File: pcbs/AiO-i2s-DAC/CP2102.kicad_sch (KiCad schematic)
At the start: 12 parts, among them U3 CP2102-GM

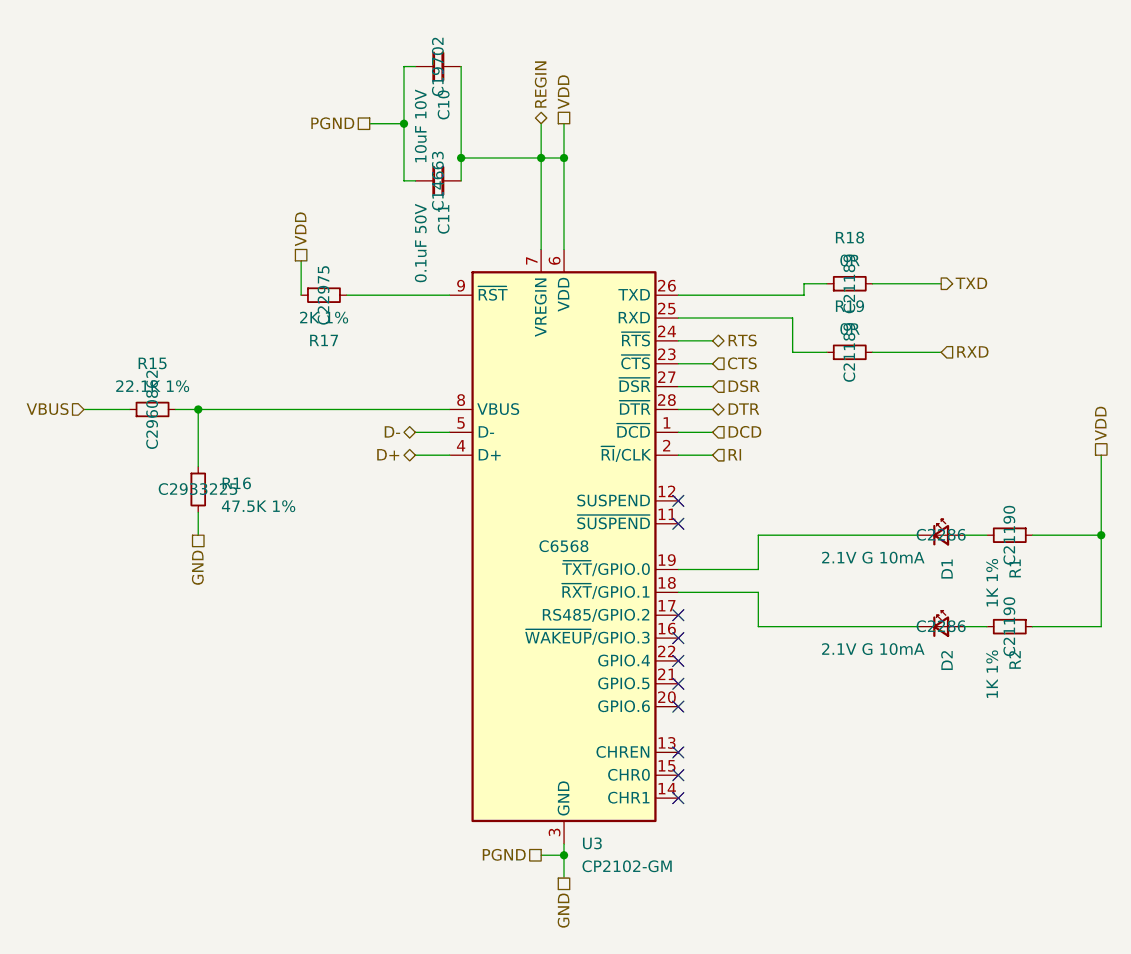
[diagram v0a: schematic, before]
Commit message: LCSC BOM Preparation
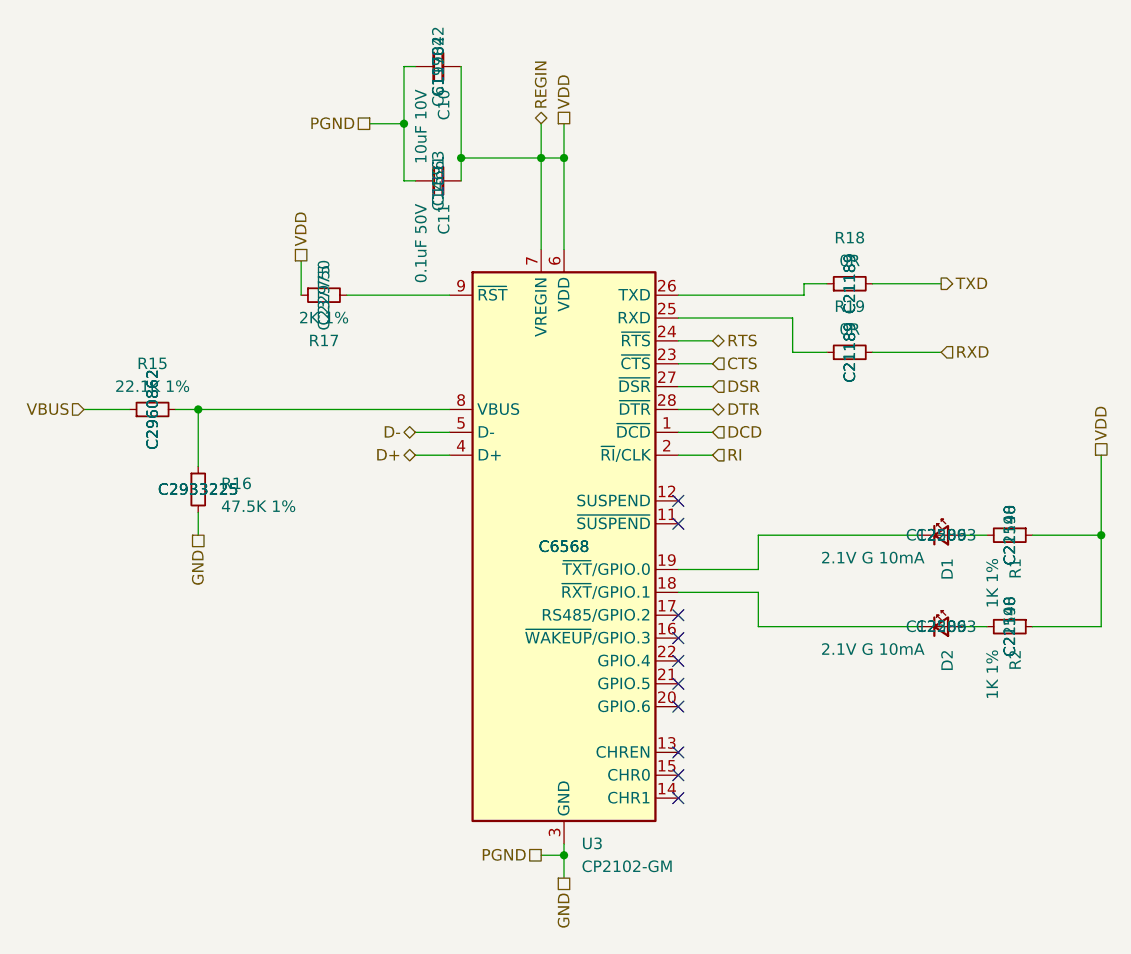
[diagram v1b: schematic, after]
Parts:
- C10: LCSC alt (none) -> C6119842
- C11: LCSC alt (none) -> C1591
- D1, D2: LCSC alt (none) -> C125093
- R1, R2: LCSC alt (none) -> C22548
- R15: LCSC alt (none) -> C2960862
- R16: LCSC alt (none) -> C2933225
- R17: LCSC alt (none) -> C237750
- R18, R19: LCSC alt (none) -> C21189
- U3: LCSC alt (none) -> C6568
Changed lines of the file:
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@@
+			)
+		)
+		(property "LCSC alt" "C22548"
+			(at 203.2 100.33 0)
+			(effects
+				(font
+					(size 1.27 1.27)
+				)
 			)
 		)
@@
 			)
 		)
+		(property "LCSC alt" "C1591"
+			(at 139.7 60.96 0)
+			(effects
+				(font
+					(size 1.27 1.27)
+				)
+			)
+		)
 		(pin "1"
 		)
@@
 			)
 		)
+		(property "LCSC alt" "C125093"
+			(at 195.58 110.49 0)
+			(effects
+				(font
+					(size 1.27 1.27)
+				)
+			)
+		)
 		(pin "1"
 		)
@@
 		)
 		(property "LCSC" "C2286"
+			(at 195.58 100.33 0)
+			(effects
+				(font
+					(size 1.27 1.27)
+				)
+			)
+		)
+		(property "LCSC alt" "C125093"
 			(at 195.58 100.33 0)
 			(effects
@@
 			)
 		)
+		(property "LCSC alt" "C21189"
+			(at 185.42 80.01 0)
+			(effects
+				(font
+					(size 1.27 1.27)
+				)
+			)
+		)
 		(pin "1"
 		)
@@
 			)
 		)
+		(property "LCSC alt" "C6119842"
+			(at 139.7 48.26 0)
+			(effects
+				(font
+					(size 1.27 1.27)
+				)
+			)
+		)
 		(pin "1"
 		)
@@
 			)
 		)
+		(property "LCSC alt" "C2960862"
+			(at 107.95 86.36 0)
+			(effects
+				(font
+					(size 1.27 1.27)
+				)
+			)
+		)
 		(pin "1"
 		)
@@
 			)
 		)
+		(property "LCSC alt" "C22548"
+			(at 203.2 110.49 0)
+			(effects
+				(font
+					(size 1.27 1.27)
+				)
+			)
+		)
 		(pin "1"
 		)
@@
 			)
 		)
+		(property "LCSC alt" "C21189"
+			(at 185.42 72.39 0)
+			(effects
+				(font
+					(size 1.27 1.27)
+				)
+			)
+		)
 		(pin "1"
 		)
@@
 			)
 		)
+		(property "LCSC alt" "C237750"
+			(at 127 73.66 0)
+			(effects
+				(font
+					(size 1.27 1.27)
+				)
+			)
+		)
 		(pin "1"
 		)
@@
 			)
 		)
+		(property "LCSC alt" "C2933225"
+			(at 113.03 95.25 0)
+			(effects
+				(font
+					(size 1.27 1.27)
+				)
+			)
+		)
 		(pin "1"
 		)
@@
 			(at 153.67 101.6 0)
 			(effects
+				(font
+					(size 1.27 1.27)
+				)
+			)
+		)
+		(property "LCSC alt" "C6568"
+			(at 153.67 101.6 0)
+			(effects

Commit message: Build prep
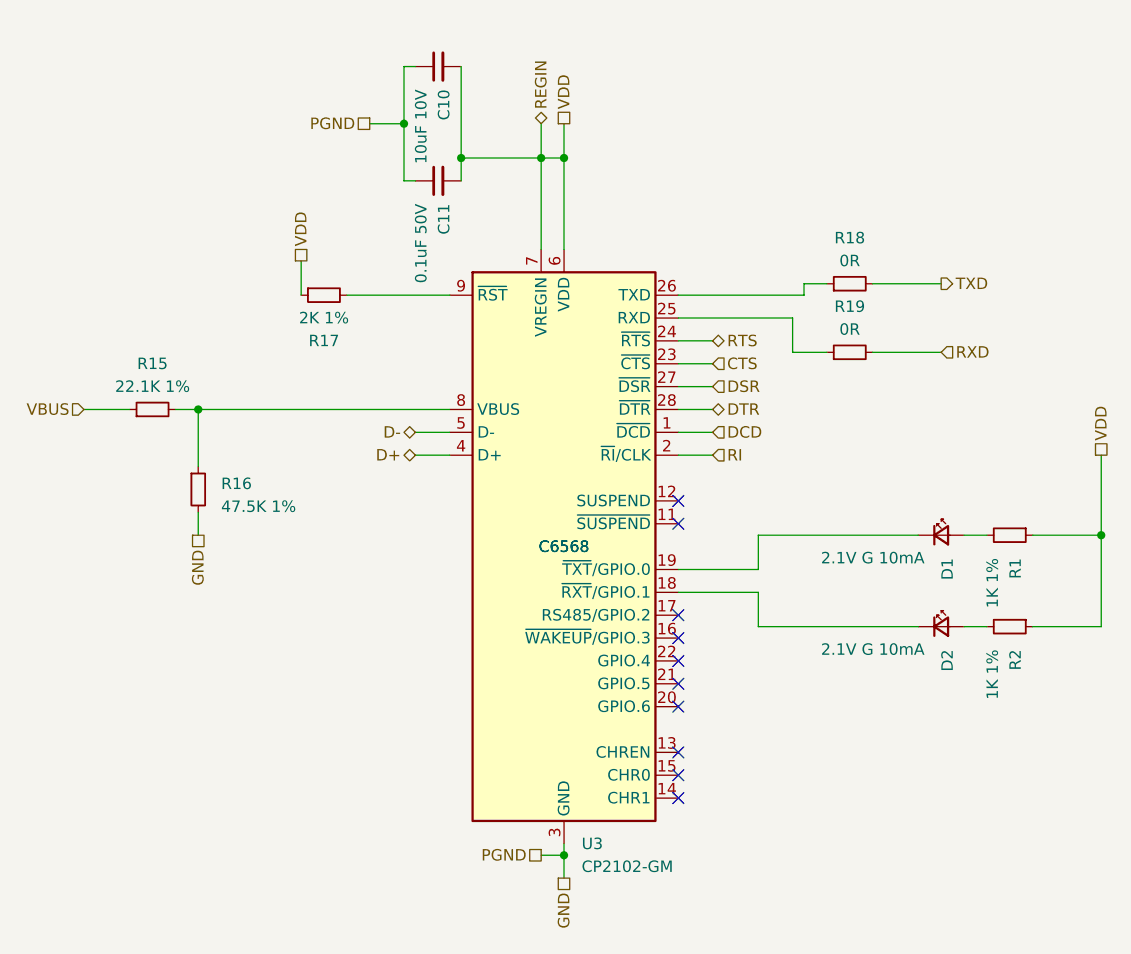
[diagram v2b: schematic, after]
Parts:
- R15: LCSC C2960862 -> C6397988
- R16: LCSC C2933225 -> C403243
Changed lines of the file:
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@@
 					(size 1.27 1.27)
 				)
+				(hide yes)
 			)
 		)
@@
 					(size 1.27 1.27)
 				)
+				(hide yes)
 			)
 		)
@@
 					(size 1.27 1.27)
 				)
+				(hide yes)
 			)
 		)
@@
 					(size 1.27 1.27)
 				)
+				(hide yes)
 			)
 		)
@@
 					(size 1.27 1.27)
 				)
+				(hide yes)
 			)
 		)
@@
 					(size 1.27 1.27)
 				)
+				(hide yes)
 			)
 		)
@@
 					(size 1.27 1.27)
 				)
+				(hide yes)
 			)
 		)
@@
 					(size 1.27 1.27)
 				)
+				(hide yes)
 			)
 		)
@@
 					(size 1.27 1.27)
 				)
+				(hide yes)
 			)
 		)
@@
 					(size 1.27 1.27)
 				)
+				(hide yes)
 			)
 		)
@@
 					(size 1.27 1.27)
 				)
+				(hide yes)
 			)
 		)
@@
 					(size 1.27 1.27)
 				)
+				(hide yes)
 			)
 		)
@@
 			)
 		)
-		(property "LCSC" "C2960862"
+		(property "LCSC" "C6397988"
 			(at 107.95 86.36 0)
 			(effects
@@
 					(size 1.27 1.27)
 				)
+				(hide yes)
 			)
 		)
@@
 					(size 1.27 1.27)
 				)
+				(hide yes)
 			)
 		)
@@
 					(size 1.27 1.27)
 				)
+				(hide yes)
 			)
 		)
@@
 					(size 1.27 1.27)
 				)
+				(hide yes)
 			)
 		)
@@
 					(size 1.27 1.27)
 				)
+				(hide yes)
 			)
 		)
@@
 					(size 1.27 1.27)
 				)
+				(hide yes)
 			)
 		)
@@
 					(size 1.27 1.27)
 				)
+				(hide yes)
 			)
 		)
@@
 					(size 1.27 1.27)
 				)
+				(hide yes)
 			)
 		)
@@
 			)
 		)
-		(property "LCSC" "C2933225"
+		(property "LCSC" "C403243"
 			(at 113.03 95.25 0)
 			(effects
@@
 					(size 1.27 1.27)
 				)
+				(hide yes)
 			)
 		)
@@
 					(size 1.27 1.27)
 				)
-			)
-		)
+				(hide yes)
+			)
+		)
